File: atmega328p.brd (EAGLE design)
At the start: 100 x 80 mm, 8 parts, among them IC1 ATMEGA328-20P, X1 CRYSTALS-NOGND-HC49

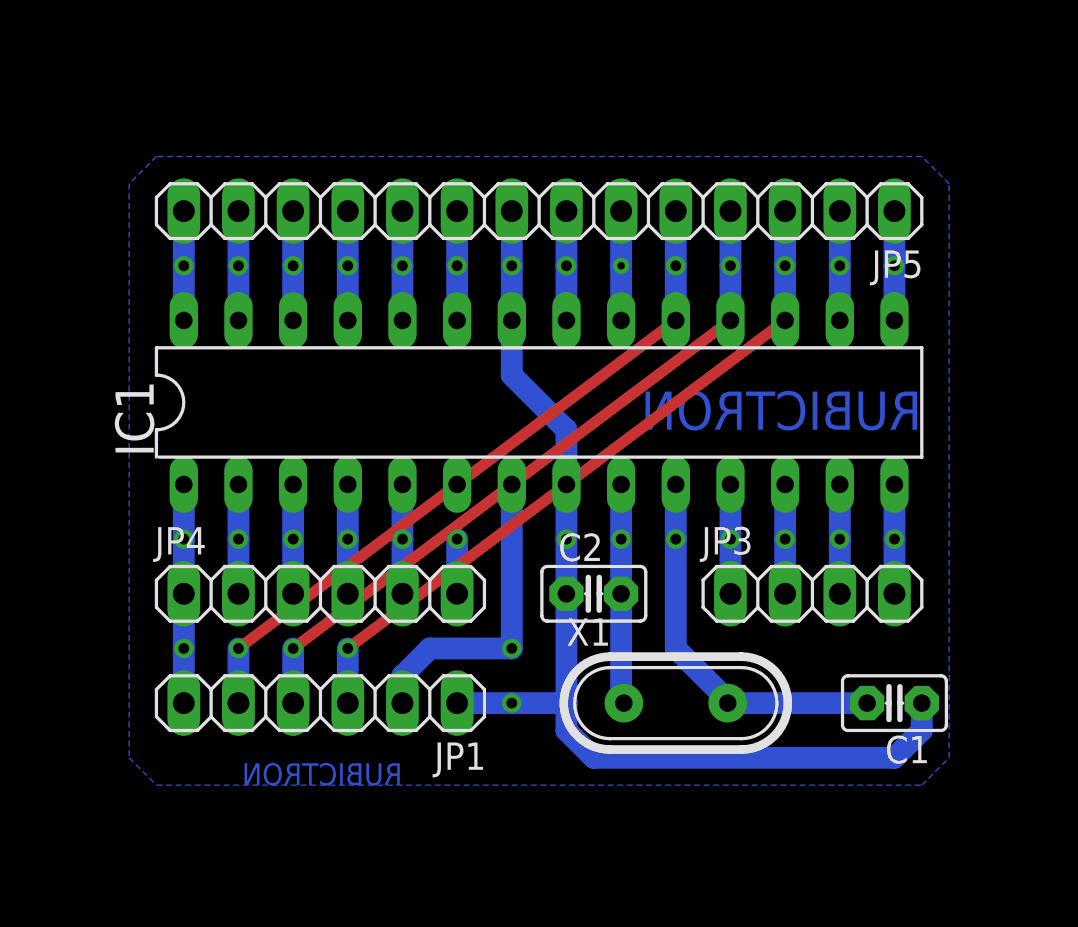
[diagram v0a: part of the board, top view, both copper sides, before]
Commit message: with pdf
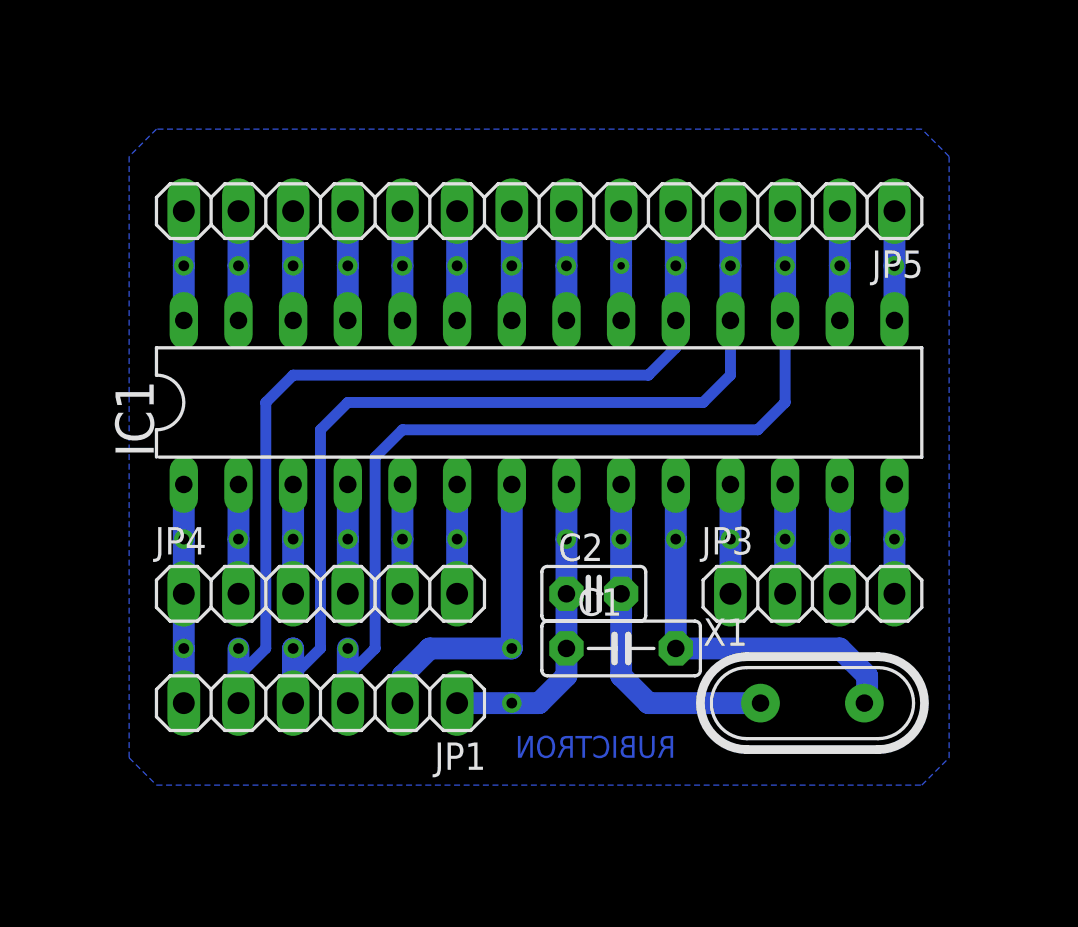
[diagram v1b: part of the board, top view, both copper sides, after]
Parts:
- C1: device capacitor-wima:C2.5-2 -> capacitor-wima:C5B2.5
- moved C1 13.0 mm to (43.2, 35.6), turned to 0 degrees
- moved X1 6.35 mm to (52.1, 33.0)
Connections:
- new net N$30: IC1.22, JP5.8
- net N$13: now also IC1.6
- net N$5: no longer IC1.22, JP5.8
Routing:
- net N$5: track 49.1 -> 14.5 mm, vias 4 -> 3
- net N$31: track 33.0 -> 43.5 mm
- net N$8: track 33.0 -> 43.5 mm
- net N$10: track 33.0 -> 42.2 mm
- net N$3: track 10.3 -> 15.9 mm
- net N$30: track 0.00 -> 5.08 mm, vias 0 -> 1
- net N$13: track 2.54 -> 5.08 mm
- net N$4: track 17.6 -> 18.4 mm
